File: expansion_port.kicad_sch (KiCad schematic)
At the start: 1 part, among them J2 Conn_02x30_Odd_Even

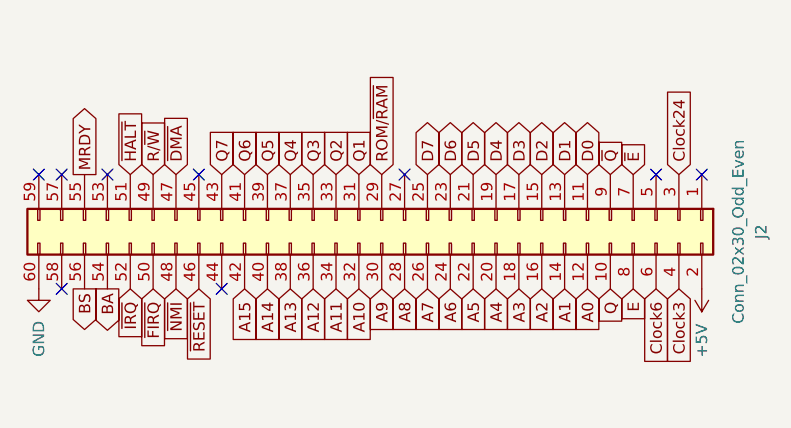
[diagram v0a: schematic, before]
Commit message: rearrange components for routing
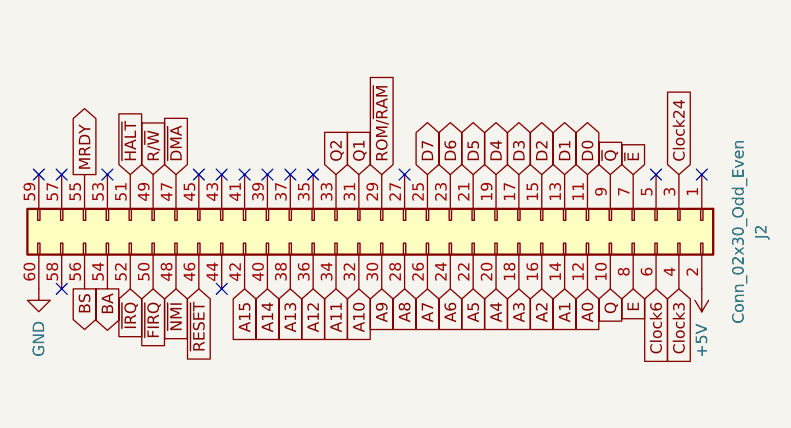
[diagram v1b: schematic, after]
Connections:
- net Q3: no longer names the net of J2.35 (Pin_35)
- net Q4: no longer names the net of J2.37 (Pin_37)
- net Q5: no longer names the net of J2.39 (Pin_39)
- net Q6: no longer names the net of J2.41 (Pin_41)
- net Q7: no longer names the net of J2.43 (Pin_43)
- no-connect marks 9 -> 14
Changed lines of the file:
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@@
   (no_connect (at 78.994 36.576))
   (no_connect (at 56.134 36.576))
+  (no_connect (at 66.294 36.576))
+  (no_connect (at 68.834 36.576))
+  (no_connect (at 58.674 36.576))
+  (no_connect (at 61.214 36.576))
+  (no_connect (at 63.754 36.576))
   (no_connect (at 45.974 36.576))
   (no_connect (at 106.934 36.576))
@@
     )
   )
-  (global_label "Q6" (shape input) (at 61.214 36.576 90) (fields_autoplaced)
-    (effects (font (size 1.27 1.27)) (justify left))
-    (property "Intersheet References" "${INTERSHEET_REFS}" (id 0) (at 61.2934 31.6229 90)
-      (effects (font (size 1.27 1.27)) (justify left) hide)
-    )
-  )
   (global_label "~{E}" (shape input) (at 104.394 36.576 90) (fields_autoplaced)
     (effects (font (size 1.27 1.27)) (justify left))
@@
     )
   )
-  (global_label "Q5" (shape input) (at 63.754 36.576 90) (fields_autoplaced)
-    (effects (font (size 1.27 1.27)) (justify left))
-    (property "Intersheet References" "${INTERSHEET_REFS}" (id 0) (at 63.8334 31.6229 90)
-      (effects (font (size 1.27 1.27)) (justify left) hide)
-    )
-  )
   (global_label "~{DMA}" (shape input) (at 53.594 36.576 90) (fields_autoplaced)
     (effects (font (size 1.27 1.27)) (justify left))
@@
     )
   )
-  (global_label "Q3" (shape input) (at 68.834 36.576 90) (fields_autoplaced)
-    (effects (font (size 1.27 1.27)) (justify left))
-    (property "Intersheet References" "${INTERSHEET_REFS}" (id 0) (at 68.9134 31.6229 90)
-      (effects (font (size 1.27 1.27)) (justify left) hide)
-    )
-  )
   (global_label "~{NMI}" (shape input) (at 53.594 49.276 270) (fields_autoplaced)
     (effects (font (size 1.27 1.27)) (justify right))
@@
     )
   )
-  (global_label "Q4" (shape input) (at 66.294 36.576 90) (fields_autoplaced)
-    (effects (font (size 1.27 1.27)) (justify left))
-    (property "Intersheet References" "${INTERSHEET_REFS}" (id 0) (at 66.3734 31.6229 90)
-      (effects (font (size 1.27 1.27)) (justify left) hide)
-    )
-  )
   (global_label "A13" (shape input) (at 66.294 49.276 270) (fields_autoplaced)
     (effects (font (size 1.27 1.27)) (justify right))
@@
       (effects (font (size 1.27 1.27)) (justify left) hide)
     )
-  )
-  (global_label "Q7" (shape input) (at 58.674 36.576 90) (fields_autoplaced)
-    (effects (font (size 1.27 1.27)) (justify left))
-    (property "Intersheet References" "${INTERSHEET_REFS}" (id 0) (at 58.7534 31.6229 90)
-      (effects (font (size 1.27 1.27)) (justify left) hide)
-    )
